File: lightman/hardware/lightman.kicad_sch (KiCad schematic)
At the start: 1 part

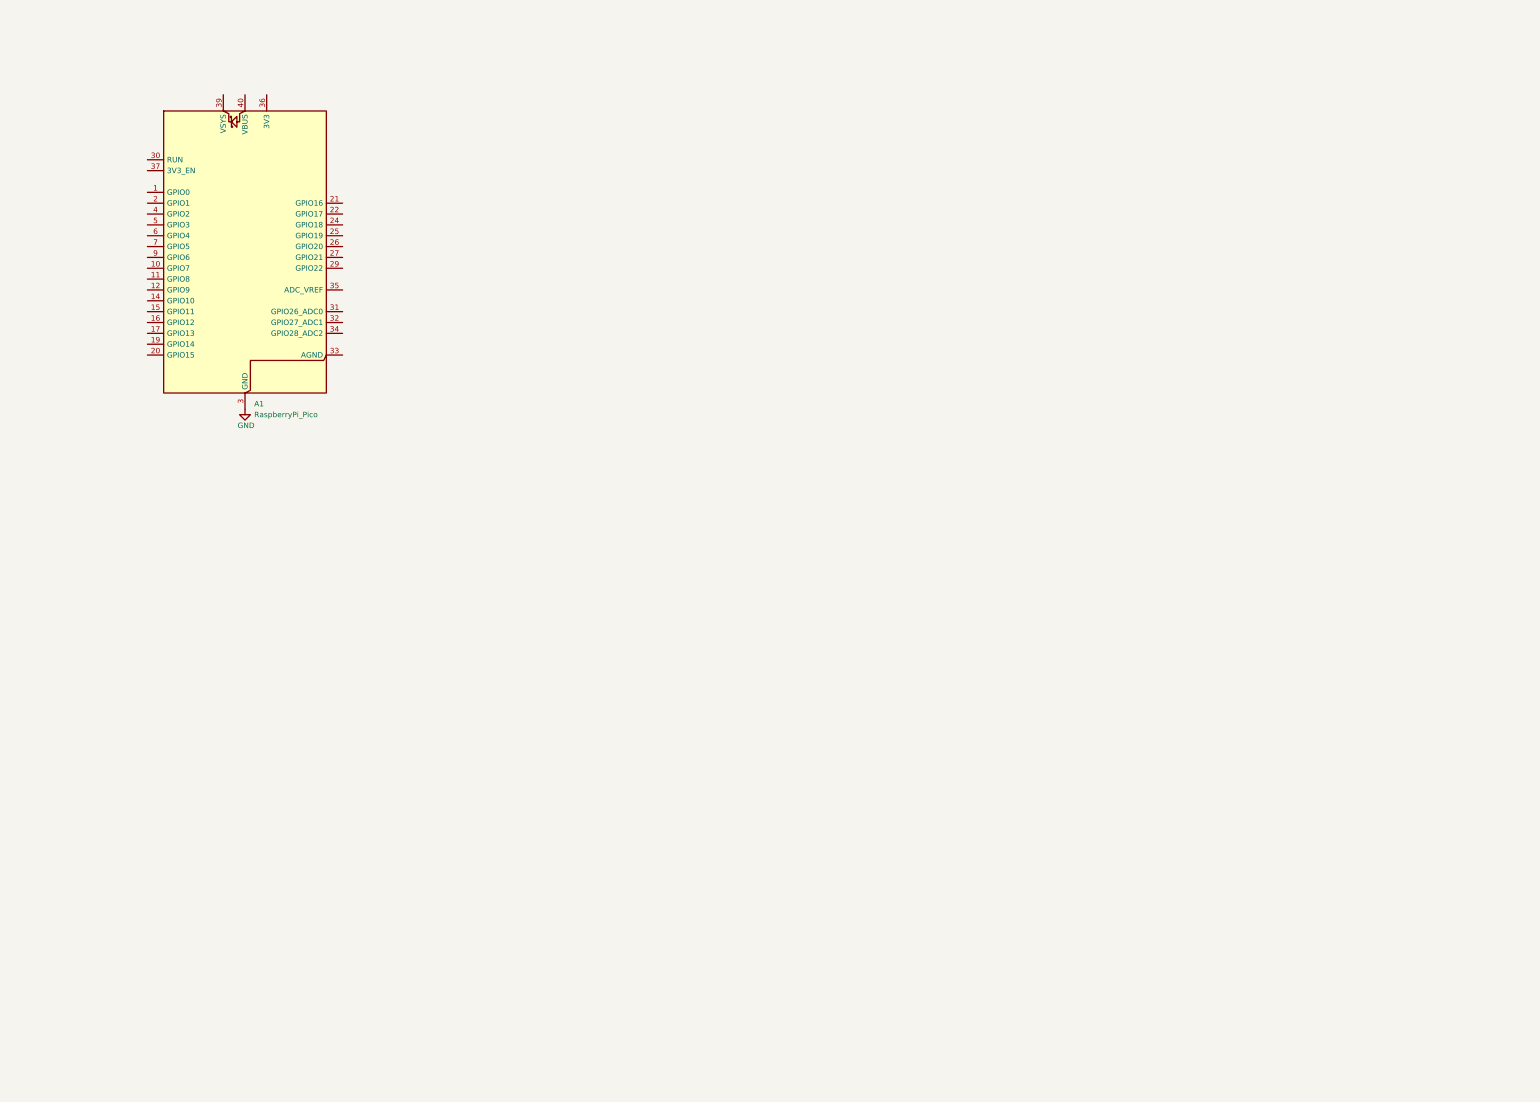
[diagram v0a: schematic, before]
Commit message: lightman source
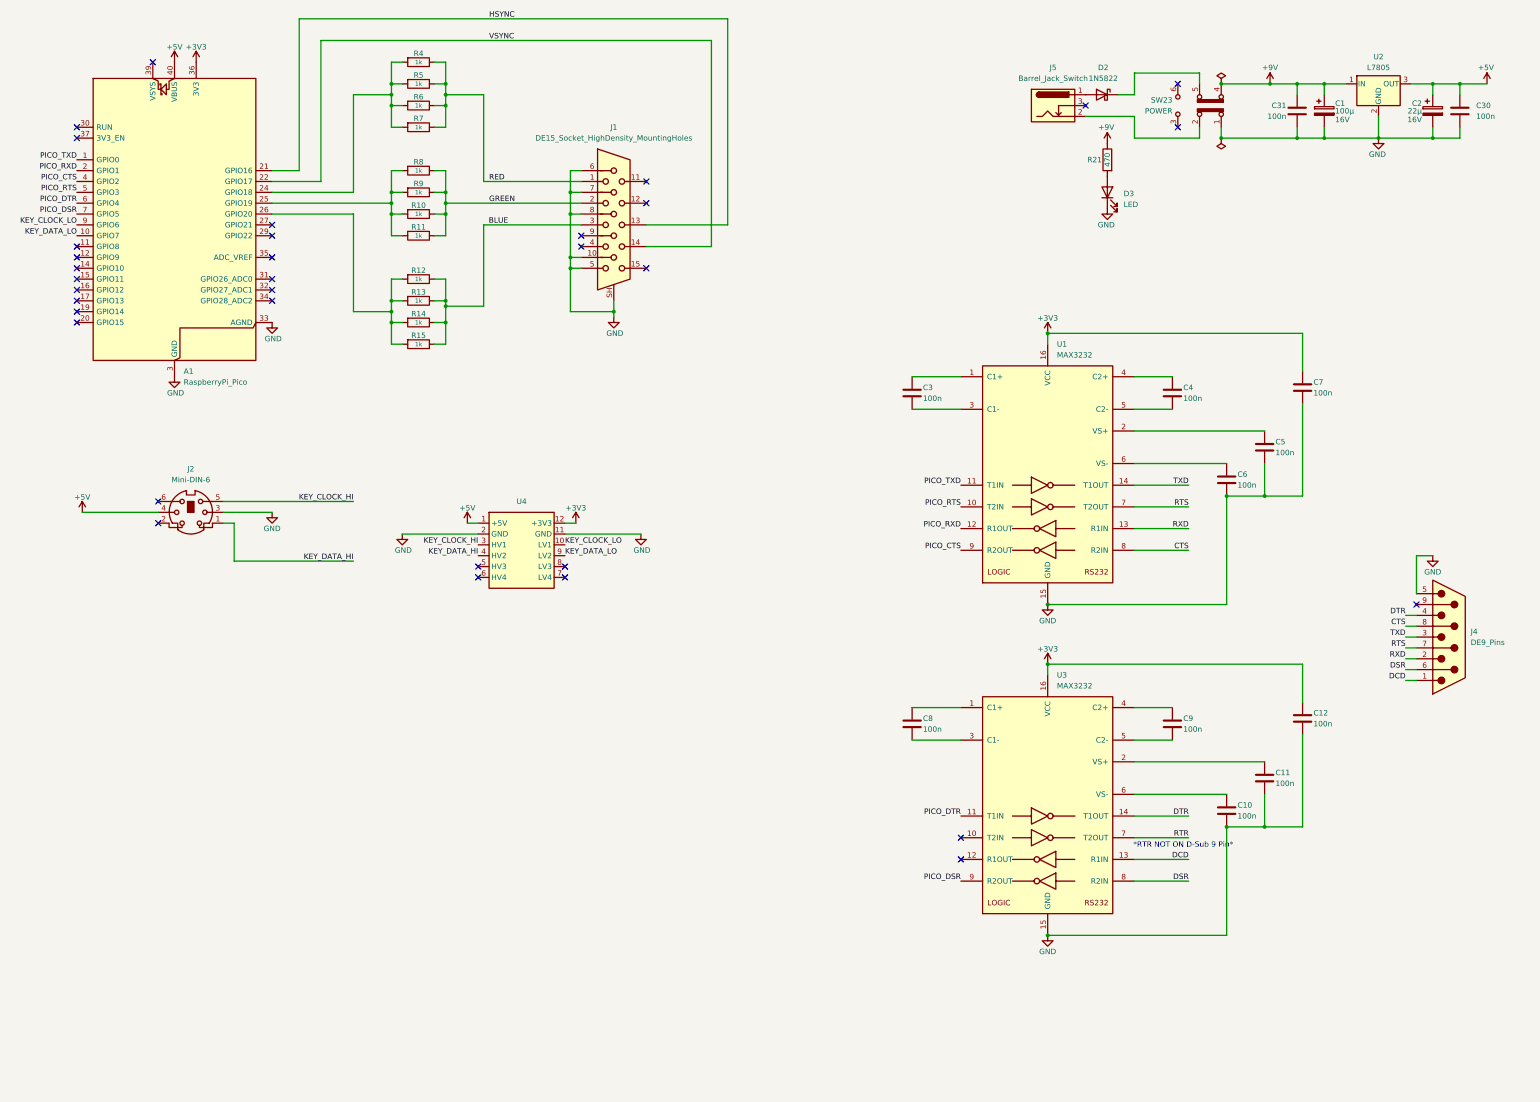
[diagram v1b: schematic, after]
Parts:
- added C1: 100µ, Capacitor_THT:CP_Radial_D6.3mm_P2.50mm, symbol Device:C_Polarized
- added C10, C11, C12, C3, C4, C5, C6, C7, C8, C9: 100n, IMNOTWOPR:C_Rect_P200mil, symbol IMNOTWOPR:C
- added C2: 22µ, Capacitor_THT:CP_Radial_D5.0mm_P2.50mm, symbol Device:C_Polarized
- added C30, C31: 100n, Desval27:C_Disc_D5.0mm_W2.5mm_P200mil, symbol Desval27:C
- added D2: 1N5822, Diode_THT:D_DO-201AD_P15.24mm_Horizontal, symbol Diode:1N5822
- added D3: LED, LED_THT:LED_D5.0mm, symbol Device:LED
- added J1: DE15_Socket_HighDensity_MountingHoles, Connector_Dsub:DSUB-15-HD_Socket_Horizontal_P2.29x2.54mm_EdgePinOffset8.35mm_Housed_MountingHolesOffset10.89mm, symbol Connector:DE15_Socket_HighDensity_MountingHoles
- added J2: Mini-DIN-6, IMNOTWOPR:KMDGX6SBS, symbol Connector:Mini-DIN-6
- added J4: DE9_Pins, Connector_Dsub:DSUB-9_Pins_Horizontal_P2.77x2.54mm_EdgePinOffset9.40mm, symbol Connector:DE9_Pins
- added J5: Barrel_Jack_Switch, Connector_BarrelJack:BarrelJack_Horizontal, symbol Connector:Barrel_Jack_Switch
- added R10, R11, R12, R13, R14, R15, R4, R5, R6, R7, R8, R9: 1k, IMNOTWOPR:R_Axial_DIN0207_P400mil, symbol IMNOTWOPR:R
- added R21: 470, Desval27:R_Axial_DIN0207_400mil, symbol Desval27:R
- added SW23: POWER, Button_Switch_THT:SW_E-Switch_EG2219_DPDT_Angled, symbol Switch:SW_Slide_DPDT
- added U1, U3: MAX3232, IMNOTWOPR:DIP-16N, symbol Interface_UART:MAX3232
- added U2: L7805, Package_TO_SOT_THT:TO-220-3_Horizontal_TabDown, symbol Regulator_Linear:L7805
- added U4: (no value), IMNOTWOPR:DIP-12W, symbol IMNOTWOPR:LevelShifter
- A1: footprint Module:RaspberryPi_Pico_Common_Unspecified -> Module:RaspberryPi_Pico_Common_THT
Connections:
- net GND: now also A1.33 (AGND), C1.2, C10.2, C11.2, C12.2, C2.2, C30.2, C31.2, C5.2, C6.2, C7.2, D3.1 (K), J1.10, J1.5, J1.6, J1.7, J1.8, J1.SH, J2.3, J4.5, SW23.1 (A), U1.15 (GND), U2.2 (GND), U3.15 (GND), U4.11 (GND), U4.2 (GND)
- net PICO_TXD: now reaches A1.1 (GPIO0)
- net PICO_TXD: now also U1.11 (T1IN)
- net KEY_DATA_LO: now reaches A1.10 (GPIO7)
- net KEY_DATA_LO: now also U4.9 (LV2)
- net PICO_RXD: now reaches A1.2 (GPIO1)
- net PICO_RXD: now also U1.12 (R1OUT)
- net HSYNC: now reaches A1.21 (GPIO16)
- net HSYNC: now also J1.13
- net VSYNC: now reaches A1.22 (GPIO17)
- net VSYNC: now also J1.14
- net at A1.24 (GPIO18): now also R4.1, R5.1, R6.1, R7.1
- net at A1.25 (GPIO19): now also R10.1, R11.1, R8.1, R9.1
- net at A1.26 (GPIO20): now also R12.1, R13.1, R14.1, R15.1
- net +3V3: now reaches A1.36 (3V3)
- net +3V3: now also C12.1, C7.1, U1.16 (VCC), U3.16 (VCC), U4.12 (+3V3)
- net PICO_CTS: now reaches A1.4 (GPIO2)
- net PICO_CTS: now also U1.9 (R2OUT)
- net +5V: now reaches A1.40 (VBUS)
- net +5V: now also C2.1, C30.1, J2.4, U2.3 (OUT), U4.1 (+5V)
- net PICO_RTS: now reaches A1.5 (GPIO3)
- net PICO_RTS: now also U1.10 (T2IN)
- net PICO_DTR: now reaches A1.6 (GPIO4)
- net PICO_DTR: now also U3.11 (T1IN)
- net PICO_DSR: now reaches A1.7 (GPIO5)
- net PICO_DSR: now also U3.9 (R2OUT)
- net KEY_CLOCK_LO: now reaches A1.9 (GPIO6)
- net KEY_CLOCK_LO: now also U4.10 (LV1)
- new net: D3.2 (A), R21.2
- new net: C10.1, U3.6 (VS-)
- new net: C8.1, U3.1 (C1+)
- new net: C11.1, U3.2 (VS+)
- new net: C8.2, U3.3 (C1-)
- new net: C9.1, U3.4 (C2+)
- new net: C9.2, U3.5 (C2-)
- new net: J5.2, SW23.2 (B)
- new net: D2.1 (K), SW23.5 (B)
- new net: D2.2 (A), J5.1
- new net: C6.1, U1.6 (VS-)
- new net: C3.1, U1.1 (C1+)
- new net: C3.2, U1.3 (C1-)
- new net: C4.1, U1.4 (C2+)
- new net: C4.2, U1.5 (C2-)
- new net: C5.1, U1.2 (VS+)
- new net +9V: C1.1, C31.1, R21.1, SW23.4 (A), U2.1 (IN)
- new net BLUE: J1.3, R12.2, R13.2, R14.2, R15.2
- new net CTS: J4.8, U1.8 (R2IN)
- new net DCD: J4.1, U3.13 (R1IN)
- new net DSR: J4.6, U3.8 (R2IN)
- new net DTR: J4.4, U3.14 (T1OUT)
- new net GREEN: J1.2, R10.2, R11.2, R8.2, R9.2
- new net KEY_CLOCK_HI: J2.5, U4.3 (HV1)
- new net KEY_DATA_HI: J2.1, U4.4 (HV2)
- new net RED: J1.1, R4.2, R5.2, R6.2, R7.2
- new net RTR: U3.7 (T2OUT)
- new net RTS: J4.7, U1.7 (T2OUT)
- new net RXD: J4.2, U1.13 (R1IN)
- new net TXD: J4.3, U1.14 (T1OUT)
- no-connect marks 0 -> 34
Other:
- note added: "*RTR NOT ON D-Sub 9 Pin*"
- moved on the sheet: A1

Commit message: lightman pcb
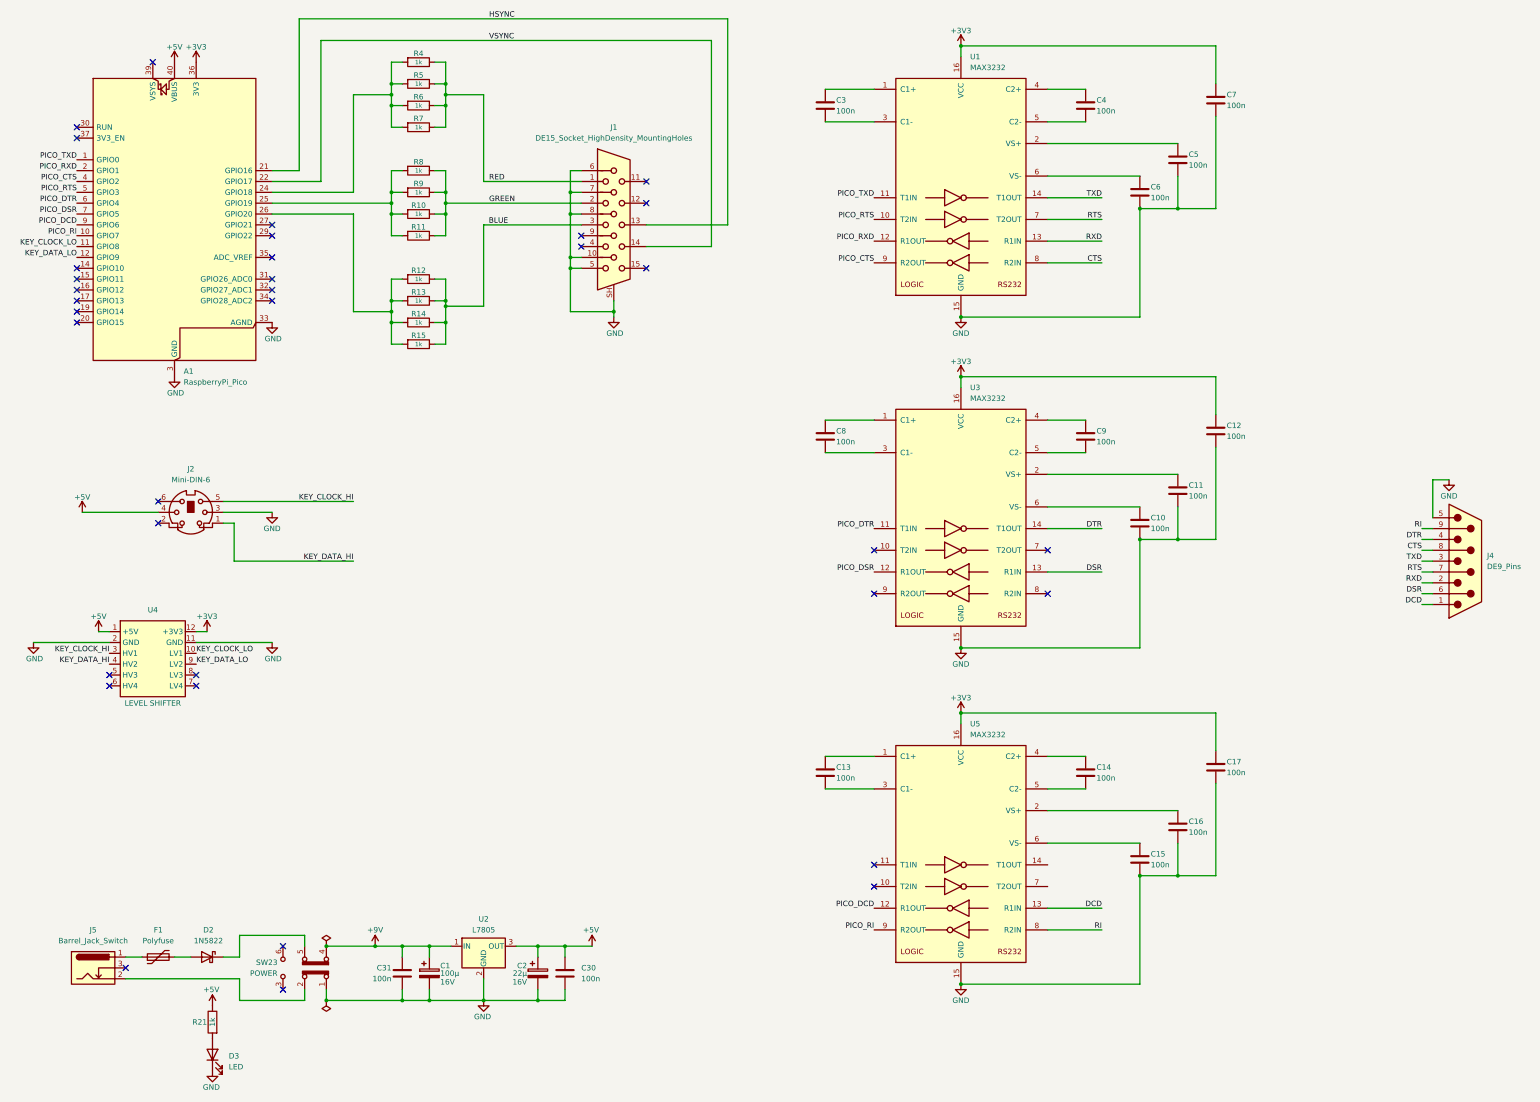
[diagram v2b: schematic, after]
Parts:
- added C13, C14, C15, C16, C17: 100n, IMNOTWOPR:C_Rect_P200mil, symbol IMNOTWOPR:C
- added F1: Polyfuse, Fuse:Fuse_Bourns_MF-RG700, symbol Device:Polyfuse
- added U5: MAX3232, IMNOTWOPR:DIP-16N, symbol Interface_UART:MAX3232
- D3: footprint LED_THT:LED_D5.0mm -> LED_THT:LED_D5.0mm_Horizontal_O1.27mm_Z3.0mm
- R21: value 470 -> 1k
- U4: value (none) -> LEVEL SHIFTER
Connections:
- net +3V3: now also C17.1, U5.16 (VCC)
- net +5V: now also R21.1
- net +9V: no longer R21.1
- net DCD: now also U5.13 (R1IN); no longer U3.13 (R1IN)
- net DSR: now also U3.13 (R1IN); no longer U3.8 (R2IN)
- net GND: now also C15.2, C16.2, C17.2, U5.15 (GND)
- net KEY_CLOCK_LO: now also A1.11 (GPIO8); no longer A1.9 (GPIO6)
- net KEY_DATA_LO: now also A1.12 (GPIO9); no longer A1.10 (GPIO7)
- net PICO_DSR: now also U3.12 (R1OUT); no longer U3.9 (R2OUT)
- net at J5.1: now also F1.1; no longer D2.2 (A)
- net RI: now reaches J4.9
- net RI: now also U5.8 (R2IN)
- net RTR: no longer names the net of U3.7 (T2OUT)
- new net: C14.1, U5.4 (C2+)
- new net: C14.2, U5.5 (C2-)
- new net: C13.1, U5.1 (C1+)
- new net: C13.2, U5.3 (C1-)
- new net: C15.1, U5.6 (VS-)
- new net: D2.2 (A), F1.2
- new net: C16.1, U5.2 (VS+)
- new net PICO_DCD: A1.9 (GPIO6), U5.12 (R1OUT)
- new net PICO_RI: A1.10 (GPIO7), U5.9 (R2OUT)
- no-connect marks 34 -> 35
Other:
- note removed: "*RTR NOT ON D-Sub 9 Pin*"
- moved on the sheet: C1, C10, C11, C12, C2, C3, C30, C31, C4, C5, C6, C7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
